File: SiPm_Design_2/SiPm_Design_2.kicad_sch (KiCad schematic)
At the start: 20 parts, among them IC1 OPA354AIDBVTG4, IC2 AFBR-S4N44P014M, IC3 AFBR-S4N44P014M, IC4 AFBR-S4N44P014M, IC5 AFBR-S4N44P014M, J3 1-1734839-0

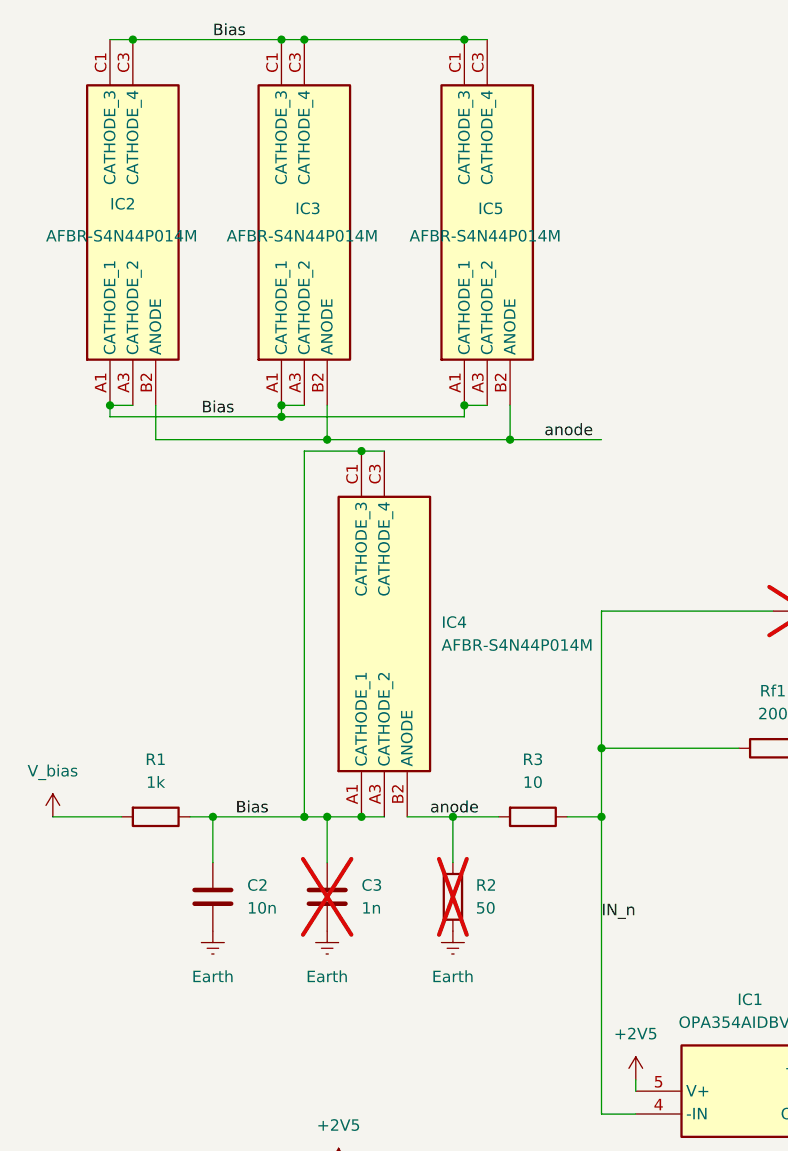
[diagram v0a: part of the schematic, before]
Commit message: update first design
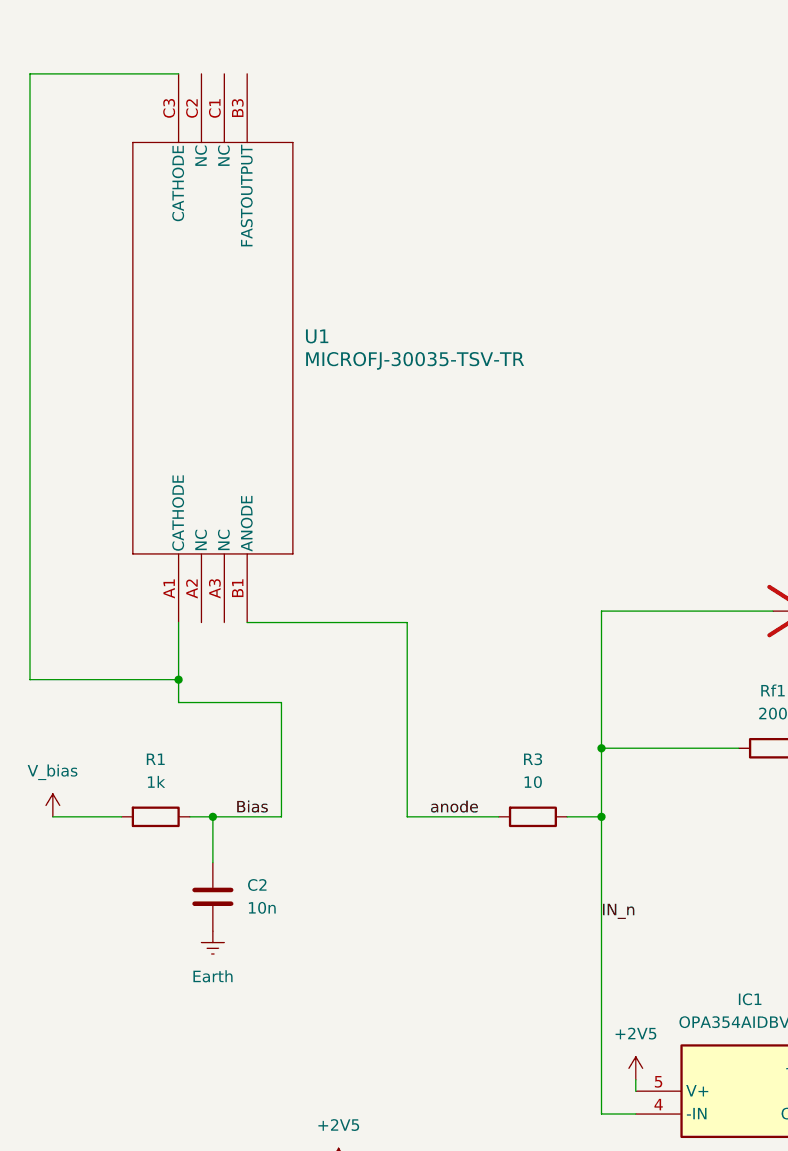
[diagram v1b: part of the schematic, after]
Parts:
- removed C3: 1n, Capacitor_SMD:C_0603_1608Metric_Pad1.08x0.95mm_HandSolder, symbol Device:C
- removed IC2, IC3, IC4, IC5: AFBR-S4N44P014M, S4N44P014M:AFBRS4N44P014M, symbol AFBR-S4N44P014M:AFBR-S4N44P014M
- removed R2: 50, Resistor_SMD:R_0603_1608Metric_Pad0.98x0.95mm_HandSolder, symbol Device:R
- added U1: MICROFJ-30035-TSV-TR, MicroFJ-300XX-TSV_ONS, symbol MICROFJ_30035_TSV_TR:MICROFJ-30035-TSV-TR
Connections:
- net Bias: now also U1.A1 (CATHODE), U1.C3 (CATHODE)
- net anode: now also U1.B1 (ANODE)

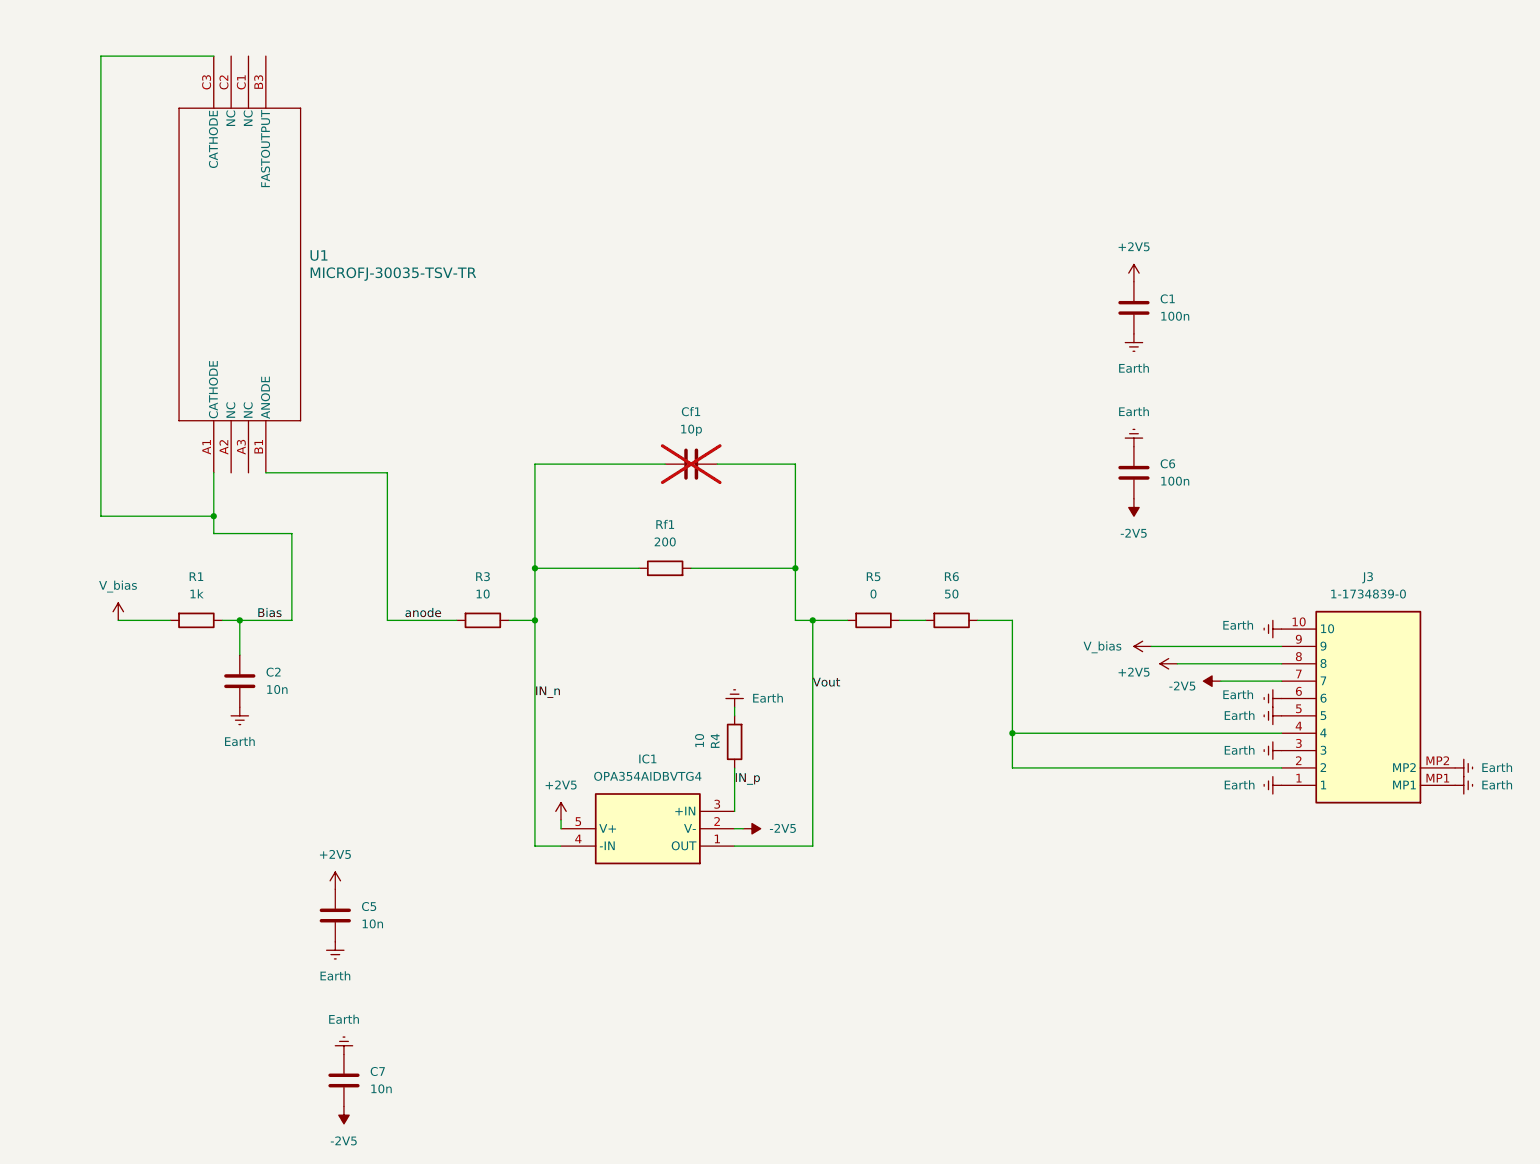
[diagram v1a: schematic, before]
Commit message: update
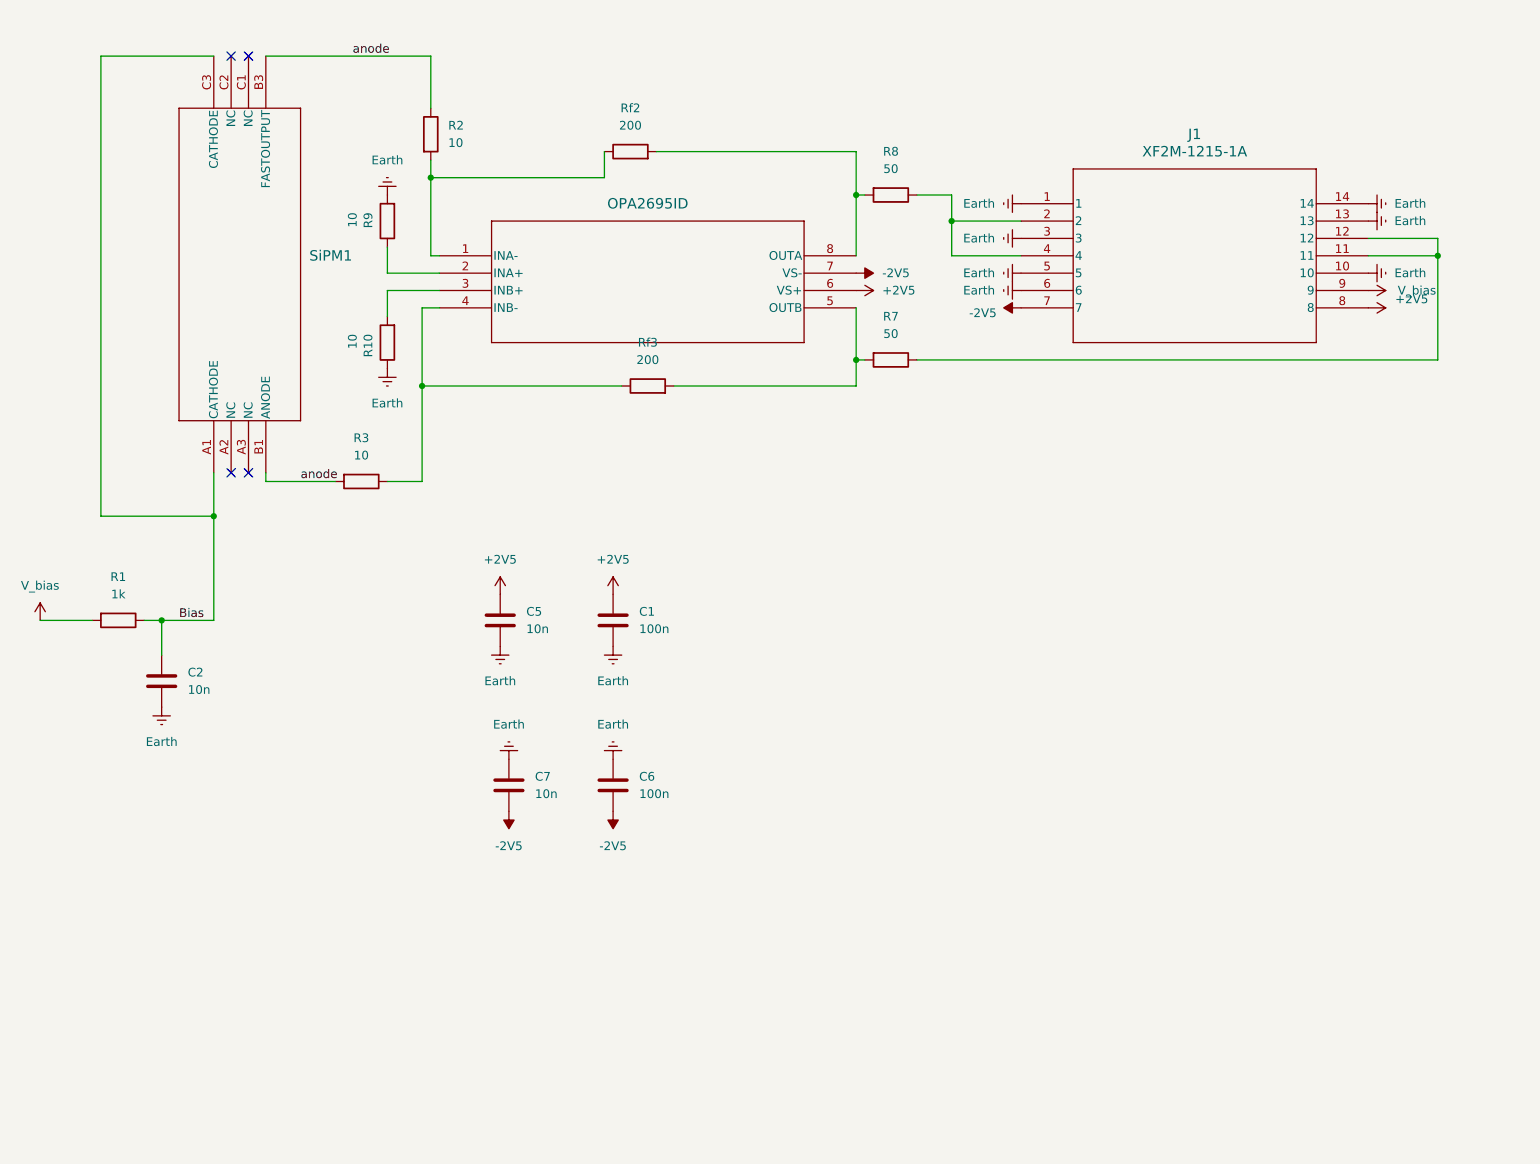
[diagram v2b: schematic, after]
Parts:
- removed Cf1: 10p, Capacitor_SMD:C_0603_1608Metric_Pad1.08x0.95mm_HandSolder, symbol Device:C
- removed IC1: OPA354AIDBVTG4, SOT95P280X145-5N, symbol OPA354AIDBVTG4:OPA354AIDBVTG4
- removed J3: 1-1734839-0, FPC 0.5 10P:117348390, symbol 1-1734839-0:1-1734839-0
- removed R4: 10, Resistor_SMD:R_0603_1608Metric_Pad0.98x0.95mm_HandSolder, symbol Device:R
- removed R5: 0, Resistor_SMD:R_0603_1608Metric_Pad0.98x0.95mm_HandSolder, symbol Device:R
- removed R6: 50, Resistor_SMD:R_0603_1608Metric_Pad0.98x0.95mm_HandSolder, symbol Device:R
- removed Rf1: 200, Resistor_SMD:R_0603_1608Metric_Pad0.98x0.95mm_HandSolder, symbol Device:R
- added J1: XF2M-1215-1A, FFC_12:CON12_1X12_DRB_XF2C_TYC, symbol FPC_12:XF2M-1215-1A
- added R10, R2, R9: 10, Resistor_SMD:R_0603_1608Metric_Pad0.98x0.95mm_HandSolder, symbol Device:R
- added R7, R8: 50, Resistor_SMD:R_0603_1608Metric_Pad0.98x0.95mm_HandSolder, symbol Device:R
- added Rf2, Rf3: 200, Resistor_SMD:R_0603_1608Metric_Pad0.98x0.95mm_HandSolder, symbol Device:R
- added U2: OPA2695ID, OPA2695:D8, symbol OPA2695:OPA2695ID
- renumbered U1 to SiPM1
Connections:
- net +2V5: now also J1.8, U2.6 (VS+)
- net -2V5: now also J1.7, U2.7 (VS-)
- net Earth: now also J1.1, J1.10, J1.13, J1.14, J1.3, J1.5, J1.6, R10.1, R9.2
- net V_bias: now also J1.9
- net anode: now also SiPM1.B3 (FASTOUTPUT), R2.1
- net IN_n: no longer names the net of R3.1
- net IN_n: now also Rf3.1, U2.4 (INB-)
- new net: R2.2, Rf2.1, U2.1 (INA-)
- new net: R8.2, Rf2.2, U2.8 (OUTA)
- new net: R9.1, U2.2 (INA+)
- new net: J1.2, J1.4, R8.1
- new net: R7.2, Rf3.2, U2.5 (OUTB)
- new net: J1.11, J1.12, R7.1
- new net: R10.2, U2.3 (INB+)
- no-connect marks 0 -> 4
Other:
- moved on the sheet: C1, C2, C5, C6, C7, R1, R3
